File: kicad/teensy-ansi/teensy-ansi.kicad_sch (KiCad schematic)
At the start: 1 part

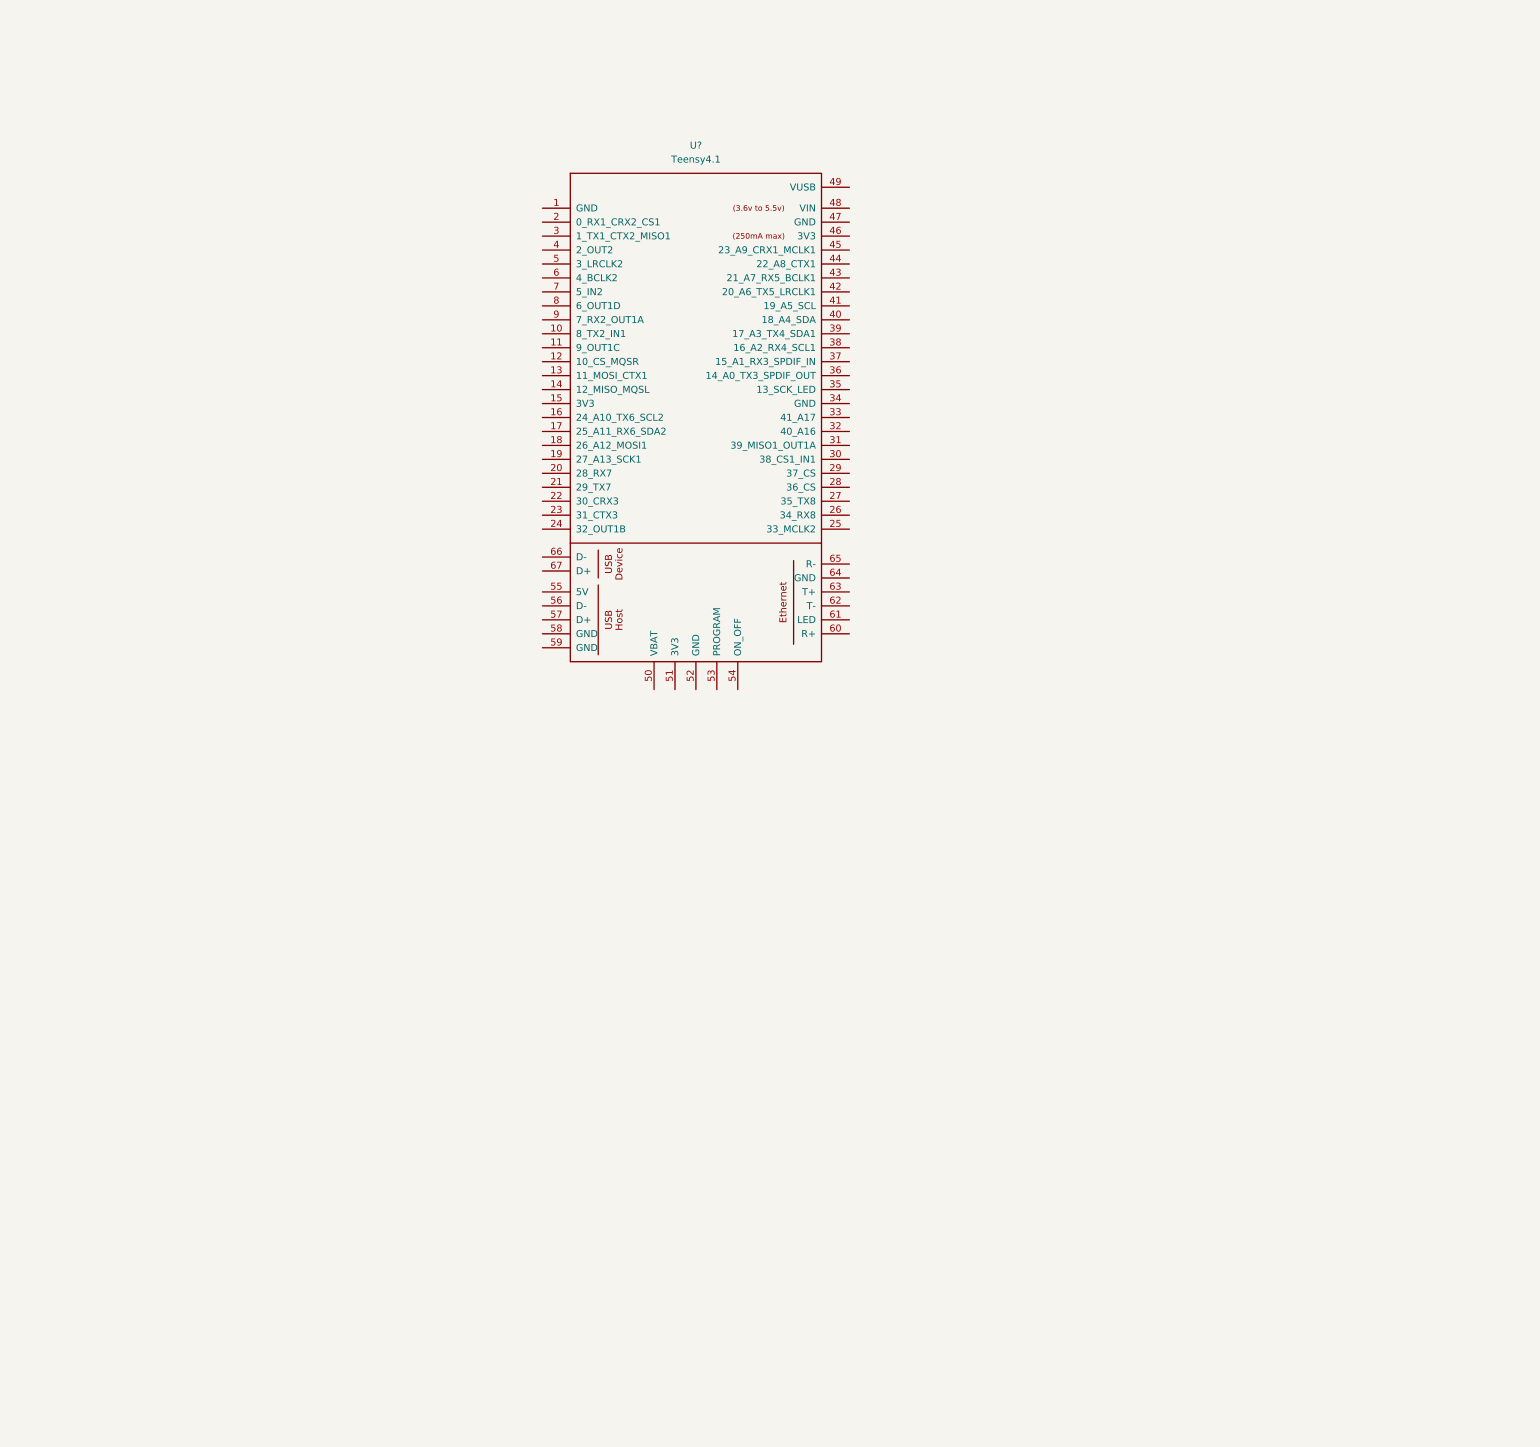
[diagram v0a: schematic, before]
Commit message: I _think_ we're nearly done with the schematic
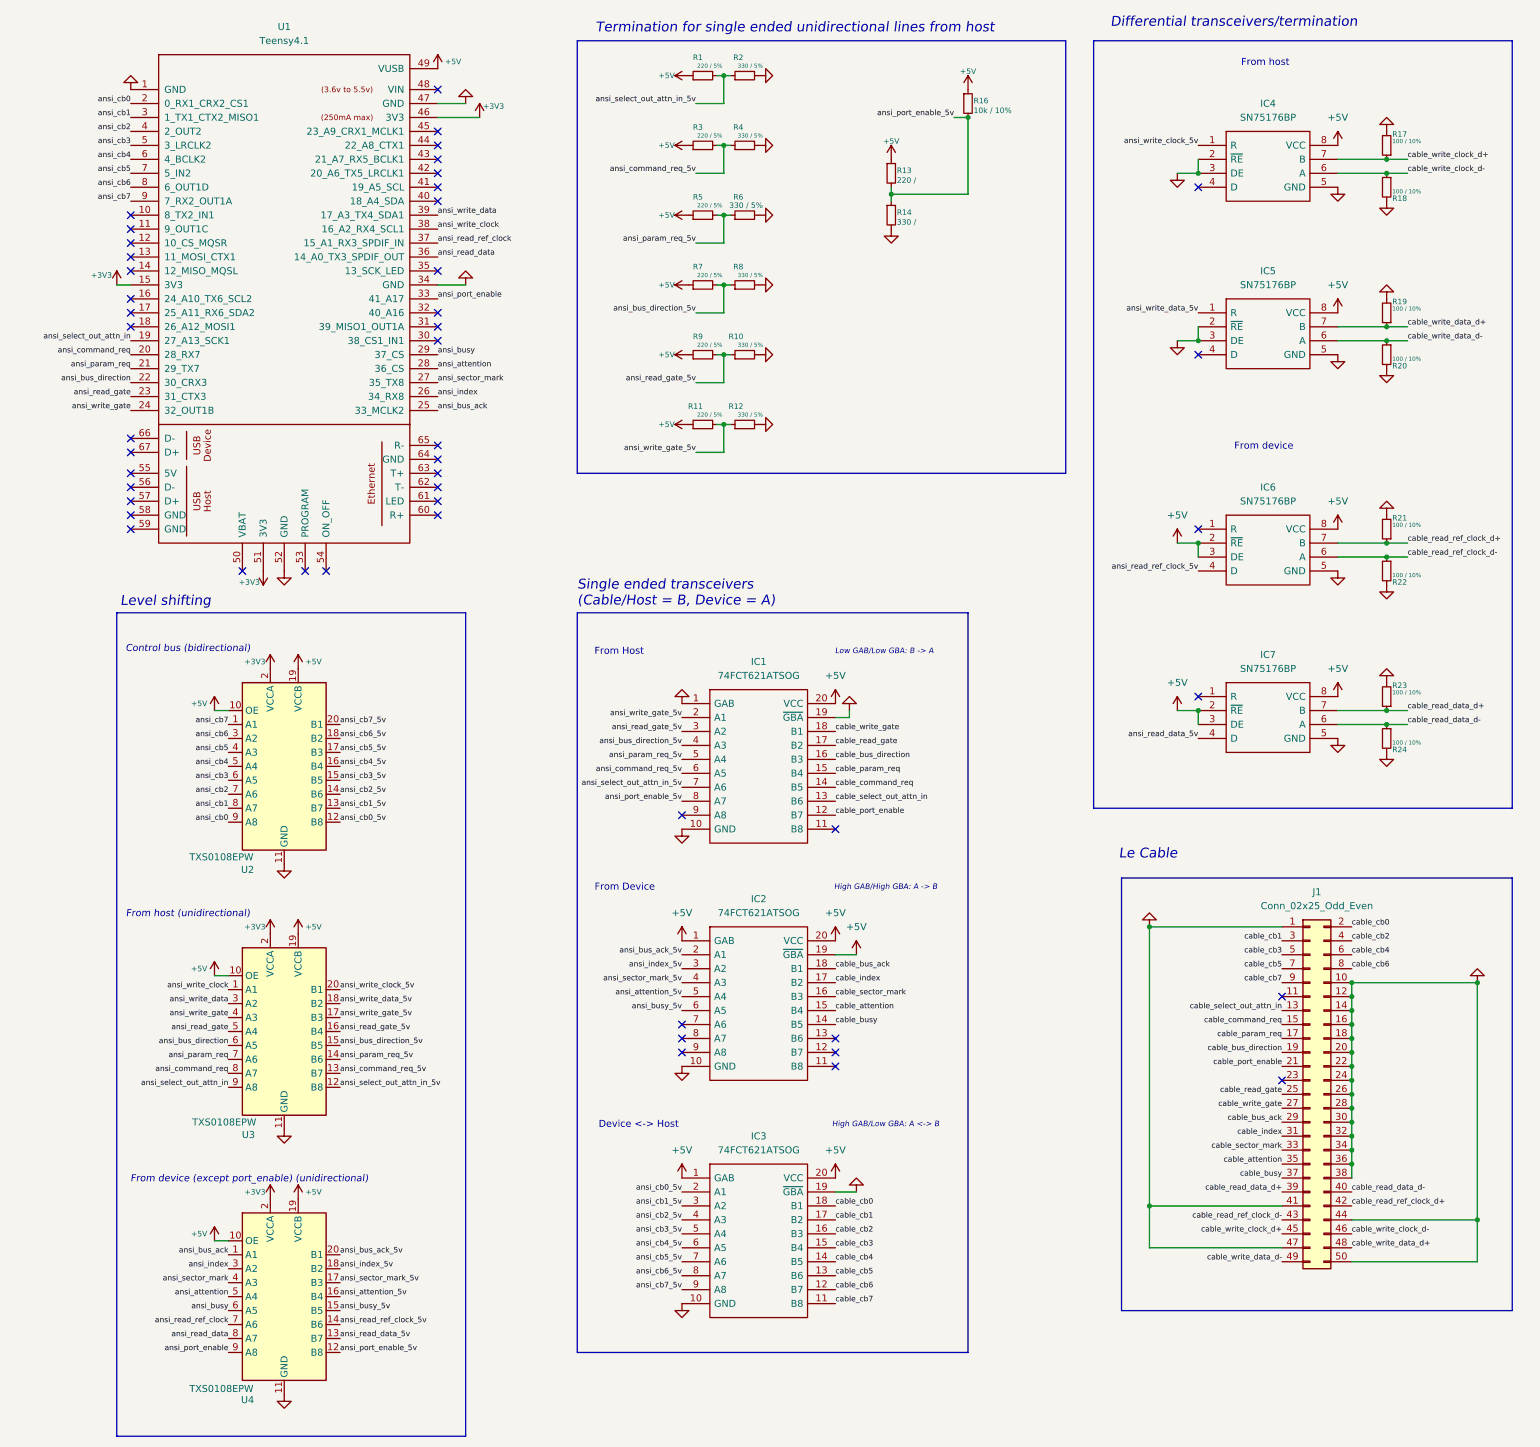
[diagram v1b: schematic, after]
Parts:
- added IC1, IC2, IC3: 74FCT621ATSOG, SOIC127P1032X265-20N, symbol 74FCT621:74FCT621ATSOG
- added IC4, IC5, IC6, IC7: SN75176BP, DIP794W53P254L959H508Q8N, symbol SN75176BP:SN75176BP
- added J1: Conn_02x25_Odd_Even, symbol Connector_Generic:Conn_02x25_Odd_Even
- added R1, R11, R3, R5, R7, R9: 220 / 5%, symbol Device:R_Small
- added R10, R12, R2, R4, R6, R8: 330 / 5%, symbol Device:R_Small
- added R13: 220 /, symbol Device:R_Small
- added R14: 330 /, symbol Device:R_Small
- added R16: 10k / 10%, symbol Device:R_Small
- added R17, R18, R19, R20, R21, R22, R23, R24: 100 / 10%, symbol Device:R_Small
- added U2, U3, U4: TXS0108EPW, Package_SO:TSSOP-20_4.4x6.5mm_P0.65mm, symbol Logic_LevelTranslator:TXS0108EPW
- gave numbers to parts that had none: 1
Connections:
- net GND: now reaches U1.1 (GND)
- net GND: now also U1.34 (GND), U1.47 (GND), U1.52 (GND), IC1.1 (GAB), IC1.10 (GND), IC1.19 (~{GBA}), IC2.10 (GND), IC3.10 (GND), IC3.19 (~{GBA}), IC4.2 (~{RE}), IC4.3 (DE), IC4.5 (GND), IC5.2 (~{RE}), IC5.3 (DE), IC5.5 (GND), IC6.5 (GND), IC7.5 (GND), J1.1 (Pin_1), J1.10 (Pin_10), J1.12 (Pin_12), J1.14 (Pin_14), J1.16 (Pin_16), J1.18 (Pin_18), J1.20 (Pin_20), J1.22 (Pin_22), J1.24 (Pin_24), J1.26 (Pin_26), J1.28 (Pin_28), J1.30 (Pin_30), J1.32 (Pin_32), J1.34 (Pin_34), J1.36 (Pin_36), J1.38 (Pin_38), J1.41 (Pin_41), J1.44 (Pin_44), J1.47 (Pin_47), J1.50 (Pin_50), R10.2, R12.2, R14.2, R17.2, R18.2, R19.2, R2.2, R20.2, R21.2, R22.2, R23.2, R24.2, R4.2, R6.2, R8.2, U2.11 (GND), U3.11 (GND), U4.11 (GND)
- net +3V3: now reaches U1.15 (3V3)
- net +3V3: now also U1.46 (3V3), U1.51 (3V3), U2.2 (VCCA), U3.2 (VCCA), U4.2 (VCCA)
- net ansi_select_out_attn_in: now reaches U1.19 (27_A13_SCK1)
- net ansi_select_out_attn_in: now also U3.9 (A8)
- net ansi_cb0: now reaches U1.2 (0_RX1_CRX2_CS1)
- net ansi_cb0: now also U2.9 (A8)
- net ansi_command_req: now reaches U1.20 (28_RX7)
- net ansi_command_req: now also U3.8 (A7)
- net ansi_param_req: now reaches U1.21 (29_TX7)
- net ansi_param_req: now also U3.7 (A6)
- net ansi_bus_direction: now reaches U1.22 (30_CRX3)
- net ansi_bus_direction: now also U3.6 (A5)
- net ansi_read_gate: now reaches U1.23 (31_CTX3)
- net ansi_read_gate: now also U3.5 (A4)
- net ansi_write_gate: now reaches U1.24 (32_OUT1B)
- net ansi_write_gate: now also U3.4 (A3)
- net ansi_bus_ack: now reaches U1.25 (33_MCLK2)
- net ansi_bus_ack: now also U4.1 (A1)
- net ansi_index: now reaches U1.26 (34_RX8)
- net ansi_index: now also U4.3 (A2)
- net ansi_sector_mark: now reaches U1.27 (35_TX8)
- net ansi_sector_mark: now also U4.4 (A3)
- net ansi_attention: now reaches U1.28 (36_CS)
- net ansi_attention: now also U4.5 (A4)
- net ansi_busy: now reaches U1.29 (37_CS)
- net ansi_busy: now also U4.6 (A5)
- net ansi_cb1: now reaches U1.3 (1_TX1_CTX2_MISO1)
- net ansi_cb1: now also U2.8 (A7)
- net ansi_port_enable: now reaches U1.33 (41_A17)
- net ansi_port_enable: now also U4.9 (A8)
- net ansi_read_data: now reaches U1.36 (14_A0_TX3_SPDIF_OUT)
- net ansi_read_data: now also U4.8 (A7)
- net ansi_read_ref_clock: now reaches U1.37 (15_A1_RX3_SPDIF_IN)
- net ansi_read_ref_clock: now also U4.7 (A6)
- net ansi_write_clock: now reaches U1.38 (16_A2_RX4_SCL1)
- net ansi_write_clock: now also U3.1 (A1)
- net ansi_write_data: now reaches U1.39 (17_A3_TX4_SDA1)
- net ansi_write_data: now also U3.3 (A2)
- net ansi_cb2: now reaches U1.4 (2_OUT2)
- net ansi_cb2: now also U2.7 (A6)
- net +5V: now reaches U1.49 (VUSB)
- net +5V: now also IC1.20 (VCC), IC2.1 (GAB), IC2.19 (~{GBA}), IC2.20 (VCC), IC3.1 (GAB), IC3.20 (VCC), IC4.8 (VCC), IC5.8 (VCC), IC6.2 (~{RE}), IC6.3 (DE), IC6.8 (VCC), IC7.2 (~{RE}), IC7.3 (DE), IC7.8 (VCC), R1.1, R11.1, R13.1, R16.1, R3.1, R5.1, R7.1, R9.1, U2.10 (OE), U2.19 (VCCB), U3.10 (OE), U3.19 (VCCB), U4.10 (OE), U4.19 (VCCB)
- net ansi_cb3: now reaches U1.5 (3_LRCLK2)
- net ansi_cb3: now also U2.6 (A5)
- net ansi_cb4: now reaches U1.6 (4_BCLK2)
- net ansi_cb4: now also U2.5 (A4)
- net ansi_cb5: now reaches U1.7 (5_IN2)
- net ansi_cb5: now also U2.4 (A3)
- net ansi_cb6: now reaches U1.8 (6_OUT1D)
- net ansi_cb6: now also U2.3 (A2)
- net ansi_cb7: now reaches U1.9 (7_RX2_OUT1A)
- net ansi_cb7: now also U2.1 (A1)
- new net ansi_attention_5v: IC2.5 (A4), U4.16 (B4)
- new net ansi_bus_ack_5v: IC2.2 (A1), U4.20 (B1)
- new net ansi_bus_direction_5v: IC1.4 (A3), R7.2, R8.1, U3.15 (B5)
- new net ansi_busy_5v: IC2.6 (A5), U4.15 (B5)
- new net ansi_cb0_5v: IC3.2 (A1), U2.12 (B8)
- new net ansi_cb1_5v: IC3.3 (A2), U2.13 (B7)
- new net ansi_cb2_5v: IC3.4 (A3), U2.14 (B6)
- new net ansi_cb3_5v: IC3.5 (A4), U2.15 (B5)
- new net ansi_cb4_5v: IC3.6 (A5), U2.16 (B4)
- new net ansi_cb5_5v: IC3.7 (A6), U2.17 (B3)
- new net ansi_cb6_5v: IC3.8 (A7), U2.18 (B2)
- new net ansi_cb7_5v: IC3.9 (A8), U2.20 (B1)
- new net ansi_command_req_5v: IC1.6 (A5), R3.2, R4.1, U3.13 (B7)
- new net ansi_index_5v: IC2.3 (A2), U4.18 (B2)
- new net ansi_param_req_5v: IC1.5 (A4), R5.2, R6.1, U3.14 (B6)
- new net ansi_port_enable_5v: IC1.8 (A7), R13.2, R14.1, R16.2, U4.12 (B8)
- new net ansi_read_data_5v: IC7.4 (D), U4.13 (B7)
- new net ansi_read_gate_5v: IC1.3 (A2), R10.1, R9.2, U3.16 (B4)
- new net ansi_read_ref_clock_5v: IC6.4 (D), U4.14 (B6)
- new net ansi_sector_mark_5v: IC2.4 (A3), U4.17 (B3)
- new net ansi_select_out_attn_in_5v: IC1.7 (A6), R1.2, R2.1, U3.12 (B8)
- new net ansi_write_clock_5v: IC4.1 (R), U3.20 (B1)
- new net ansi_write_data_5v: IC5.1 (R), U3.18 (B2)
- new net ansi_write_gate_5v: IC1.2 (A1), R11.2, R12.1, U3.17 (B3)
- new net cable_attention: IC2.15 (B4), J1.35 (Pin_35)
- new net cable_bus_ack: IC2.18 (B1), J1.29 (Pin_29)
- new net cable_bus_direction: IC1.16 (B3), J1.19 (Pin_19)
- new net cable_busy: IC2.14 (B5), J1.37 (Pin_37)
- new net cable_cb0: IC3.18 (B1), J1.2 (Pin_2)
- new net cable_cb1: IC3.17 (B2), J1.3 (Pin_3)
- new net cable_cb2: IC3.16 (B3), J1.4 (Pin_4)
- new net cable_cb3: IC3.15 (B4), J1.5 (Pin_5)
- new net cable_cb4: IC3.14 (B5), J1.6 (Pin_6)
- new net cable_cb5: IC3.13 (B6), J1.7 (Pin_7)
- new net cable_cb6: IC3.12 (B7), J1.8 (Pin_8)
- new net cable_cb7: IC3.11 (B8), J1.9 (Pin_9)
- new net cable_command_req: IC1.14 (B5), J1.15 (Pin_15)
- new net cable_index: IC2.17 (B2), J1.31 (Pin_31)
- new net cable_param_req: IC1.15 (B4), J1.17 (Pin_17)
- new net cable_port_enable: IC1.12 (B7), J1.21 (Pin_21)
- new net cable_read_data_d+: IC7.7 (B), J1.39 (Pin_39), R23.1
- new net cable_read_data_d-: IC7.6 (A), J1.40 (Pin_40), R24.1
- new net cable_read_gate: IC1.17 (B2), J1.25 (Pin_25)
- new net cable_read_ref_clock_d+: IC6.7 (B), J1.42 (Pin_42), R21.1
- new net cable_read_ref_clock_d-: IC6.6 (A), J1.43 (Pin_43), R22.1
- new net cable_sector_mark: IC2.16 (B3), J1.33 (Pin_33)
- new net cable_select_out_attn_in: IC1.13 (B6), J1.13 (Pin_13)
- new net cable_write_clock_d+: IC4.7 (B), J1.45 (Pin_45), R17.1
- new net cable_write_clock_d-: IC4.6 (A), J1.46 (Pin_46), R18.1
- new net cable_write_data_d+: IC5.7 (B), J1.48 (Pin_48), R19.1
- new net cable_write_data_d-: IC5.6 (A), J1.49 (Pin_49), R20.1
- new net cable_write_gate: IC1.18 (B1), J1.27 (Pin_27)
- no-connect marks 0 -> 49
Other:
- note added: "Control bus (bidirectional)"
- note added: "Device <-> Host"
- note added: "Differential transceivers/termination"
- note added: "From Device"
- note added: "From Host"
- note added: "From device"
- note added: "From device (except port_enable) (unidirectional)"
- note added: "From host"
- note added: "From host (unidirectional)"
- note added: "High GAB/High GBA: A -> B"
- note added: "High GAB/Low GBA: A <-> B"
- note added: "Le Cable"
- note added: "Level shifting"
- note added: "Low GAB/Low GBA: B -> A"
- note added: "Single ended transceivers (Cable/Host = B, Device = A)"
- note added: "Termination for single ended unidirectional lines from host"
- company: (none) -> Toshok Electric Light & Manufacturing
- title: (none) -> TANSI breadboard design
- moved on the sheet: U1

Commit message: biggest change is routing ansi_bus_direction_out_5v into GBA/GAB of the control bus transceiver
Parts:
- removed R10, R12, R6, R8: 330 / 5%, symbol Device:R_Small
- removed R11, R5, R7, R9: 220 / 5%, symbol Device:R_Small
- removed R13: 220 /, symbol Device:R_Small
- removed R14: 330 /, symbol Device:R_Small
- added DS1: LTA-1000E, DIPS762W50P254L2527H825Q20N, symbol LTA-1000E:LTA-1000E
- added J2: Barrel_Jack, symbol Connector:Barrel_Jack
- added R25, R26, R27, R28, R29, R30, R31, R32, R33, R34: 150 / 10%, Resistor_SMD:R_01005_0402Metric, symbol Device:R_Small
- added R? (x5): 220 / 5%, Resistor_SMD:R_01005_0402Metric, symbol Device:R_Small
- added R? (x5): 330 / %5, Resistor_SMD:R_01005_0402Metric, symbol Device:R_Small
- IC1, IC2, IC3: footprint SOIC127P1032X265-20N -> Package_SO:SOIC-20W_7.5x12.8mm_P1.27mm
- IC4, IC5, IC6, IC7: footprint DIP794W53P254L959H508Q8N -> Package_SO:SOIC-8-1EP_3.9x4.9mm_P1.27mm_EP2.95x4.9mm_Mask2.71x3.4mm
- J1: footprint (none) -> Connector_IDC:IDC-Header_2x25_P2.54mm_Vertical
- R1, R16, R17, R18, R19, R20, R21, R22, R23, R24, R3: footprint (none) -> Resistor_SMD:R_01005_0402Metric
- R2, R4: value 330 / 5% -> 330 / %5; footprint (none) -> Resistor_SMD:R_01005_0402Metric
- U1: footprint (none) -> teensy:Teensy41
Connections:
- net +5V: now also J2.2, R25.2, R?.1, R?.1, R?.1, R?.1, R?.1; no longer IC3.1 (GAB)
- net GND: now also DS1.11 (K_K), DS1.12 (K_J), DS1.13 (K_H), DS1.14 (K_G), DS1.15 (K_F), DS1.16 (K_E), DS1.17 (K_D), DS1.18 (K_C), DS1.19 (K_B), DS1.20 (K_A), J2.1, R?.2, R?.2, R?.2, R?.2, R?.2; no longer IC3.19 (~{GBA})
- net ansi_bus_direction_5v: now also IC3.1 (GAB), IC3.19 (~{GBA})
- net ansi_cb0_5v: now also IC3.9 (A8); no longer IC3.2 (A1)
- net ansi_cb1_5v: now also IC3.5 (A4), U2.16 (B4); no longer IC3.3 (A2), U2.13 (B7)
- net ansi_cb2_5v: now also IC3.8 (A7), U2.13 (B7); no longer IC3.4 (A3), U2.14 (B6)
- net ansi_cb3_5v: now also IC3.4 (A3), U2.17 (B3); no longer IC3.5 (A4), U2.15 (B5)
- net ansi_cb4_5v: now also IC3.7 (A6), U2.14 (B6); no longer IC3.6 (A5), U2.16 (B4)
- net ansi_cb5_5v: now also IC3.3 (A2), U2.18 (B2); no longer IC3.7 (A6), U2.17 (B3)
- net ansi_cb6_5v: now also IC3.6 (A5), U2.15 (B5); no longer IC3.8 (A7), U2.18 (B2)
- net ansi_cb7_5v: now also IC3.2 (A1); no longer IC3.9 (A8)
- net ansi_command_req_5v: no longer R3.2, R4.1
- net ansi_port_enable_5v: now also U4.14 (B6); no longer R16.2, U4.12 (B8)
- net ansi_read_data_5v: now also U4.12 (B8); no longer U4.13 (B7)
- net ansi_read_ref_clock_5v: now also U4.13 (B7); no longer U4.14 (B6)
- net ansi_select_out_attn_in_5v: no longer R1.2, R2.1
- net cable_bus_direction: now also R1.2, R2.1
- net cable_cb0: now also IC3.11 (B8); no longer IC3.18 (B1)
- net cable_cb1: now also IC3.15 (B4); no longer IC3.17 (B2)
- net cable_cb2: now also IC3.12 (B7); no longer IC3.16 (B3)
- net cable_cb3: now also IC3.16 (B3); no longer IC3.15 (B4)
- net cable_cb4: now also IC3.13 (B6); no longer IC3.14 (B5)
- net cable_cb5: now also IC3.17 (B2); no longer IC3.13 (B6)
- net cable_cb6: now also IC3.14 (B5); no longer IC3.12 (B7)
- net cable_cb7: now also IC3.18 (B1); no longer IC3.11 (B8)
- net cable_command_req: now also R?.1, R?.2
- net cable_param_req: now also R?.1, R?.2
- net cable_port_enable: now also R16.2, R26.2, R?.1, R?.2
- net cable_read_data_d+: now also IC7.6 (A), R24.1; no longer IC7.7 (B), R23.1
- net cable_read_data_d-: now also IC7.7 (B), R23.1; no longer IC7.6 (A), R24.1
- net cable_read_gate: now also R3.2, R4.1
- net cable_read_ref_clock_d+: now also IC6.6 (A), R22.1; no longer IC6.7 (B), R21.1
- net cable_read_ref_clock_d-: now also IC6.7 (B), R21.1; no longer IC6.6 (A), R22.1
- net cable_select_out_attn_in: now also R?.1, R?.2
- net cable_write_clock_d+: now also IC4.6 (A), R18.1; no longer IC4.7 (B), R17.1
- net cable_write_clock_d-: now also IC4.7 (B), R17.1; no longer IC4.6 (A), R18.1
- net cable_write_data_d+: now also IC5.6 (A), R20.1; no longer IC5.7 (B), R19.1
- net cable_write_data_d-: now also IC5.7 (B), R19.1; no longer IC5.6 (A), R20.1
- net cable_write_gate: now also R?.1, R?.2
- net ansi_attention renamed ansi_attention_3v
- net ansi_bus_ack renamed ansi_bus_ack_3v
- net ansi_bus_direction renamed ansi_bus_direction_3v
- net ansi_busy renamed ansi_busy_3v
- net ansi_cb0 renamed ansi_cb0_3v
- net ansi_cb1 renamed ansi_cb2_3v
- net ansi_cb2 renamed ansi_cb4_3v
- net ansi_cb3 renamed ansi_cb6_3v
- net ansi_cb4 renamed ansi_cb1_3v
- net ansi_cb5 renamed ansi_cb3_3v
- net ansi_cb6 renamed ansi_cb5_3v
- net ansi_cb7 renamed ansi_cb7_3v
- net ansi_command_req renamed ansi_command_req_3v
- net ansi_index renamed ansi_index_3v
- net ansi_param_req renamed ansi_param_req_3v
- net ansi_port_enable renamed ansi_port_enable_3v
- net ansi_port_enable_3v: now also U4.7 (A6); no longer U4.9 (A8)
- net ansi_read_data renamed ansi_read_data_3v
- net ansi_read_data_3v: now also U4.9 (A8); no longer U4.8 (A7)
- net ansi_read_gate renamed ansi_read_gate_3v
- net ansi_read_ref_clock renamed ansi_read_ref_clock_3v
- net ansi_read_ref_clock_3v: now also U4.8 (A7); no longer U4.7 (A6)
- net ansi_sector_mark renamed ansi_sector_mark_3v
- net ansi_select_out_attn_in renamed ansi_select_out_attn_in_3v
- net ansi_write_clock renamed ansi_write_clock_3v
- net ansi_write_clock_3v: now also U1.39 (17_A3_TX4_SDA1); no longer U1.38 (16_A2_RX4_SCL1)
- net ansi_write_data renamed ansi_write_data_3v
- net ansi_write_data_3v: now also U1.38 (16_A2_RX4_SCL1); no longer U1.39 (17_A3_TX4_SDA1)
- net ansi_write_gate renamed ansi_write_gate_3v
- new net: DS1.7 (A_G), R31.1
- new net: DS1.6 (A_F), R30.1
- new net: DS1.1 (A_A), R25.1
- new net: DS1.10 (A_K), R34.1
- new net: DS1.2 (A_B), R26.1
- new net: DS1.3 (A_C), R27.1
- new net: DS1.4 (A_D), R28.1
- new net: DS1.5 (A_E), R29.1
- new net: DS1.8 (A_H), R32.1
- new net: DS1.9 (A_J), R33.1
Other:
- note added: "All R = 150/10%"
- note added: "Debugging"
- note added: "Low (ACTIVE) Bus Direction Out: B -> A High (INACTIVE) Bus Direction Out: A -> B"
- note added: "Single ended transceivers / termination (Cable/Host = B, Device = A)"
- note added: "Teensy and level shifters"
- note removed: "High GAB/Low GBA: A <-> B"
- note removed: "Level shifting"
- note removed: "Single ended transceivers (Cable/Host = B, Device = A)"
- note removed: "Termination for single ended unidirectional lines from host"
- title: TANSI breadboard design -> TANSI breadboard
- moved on the sheet: IC1, IC2, IC3, IC4, IC5, IC6, IC7, J1, R16, R17, R18, R19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
